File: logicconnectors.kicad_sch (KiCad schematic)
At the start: 31 parts, among them J1 ServoConn, J1 USBC Socket, J10 LHConn, J11 MosTempConn, J12 LogicConn, J2 LogicConn2, J4 ADCConn, J5 HallConn, J6 UartSpi, J7 JTAG, J8 CANConn, U2 USBLC6-2P6, U6 TJA1051T-3

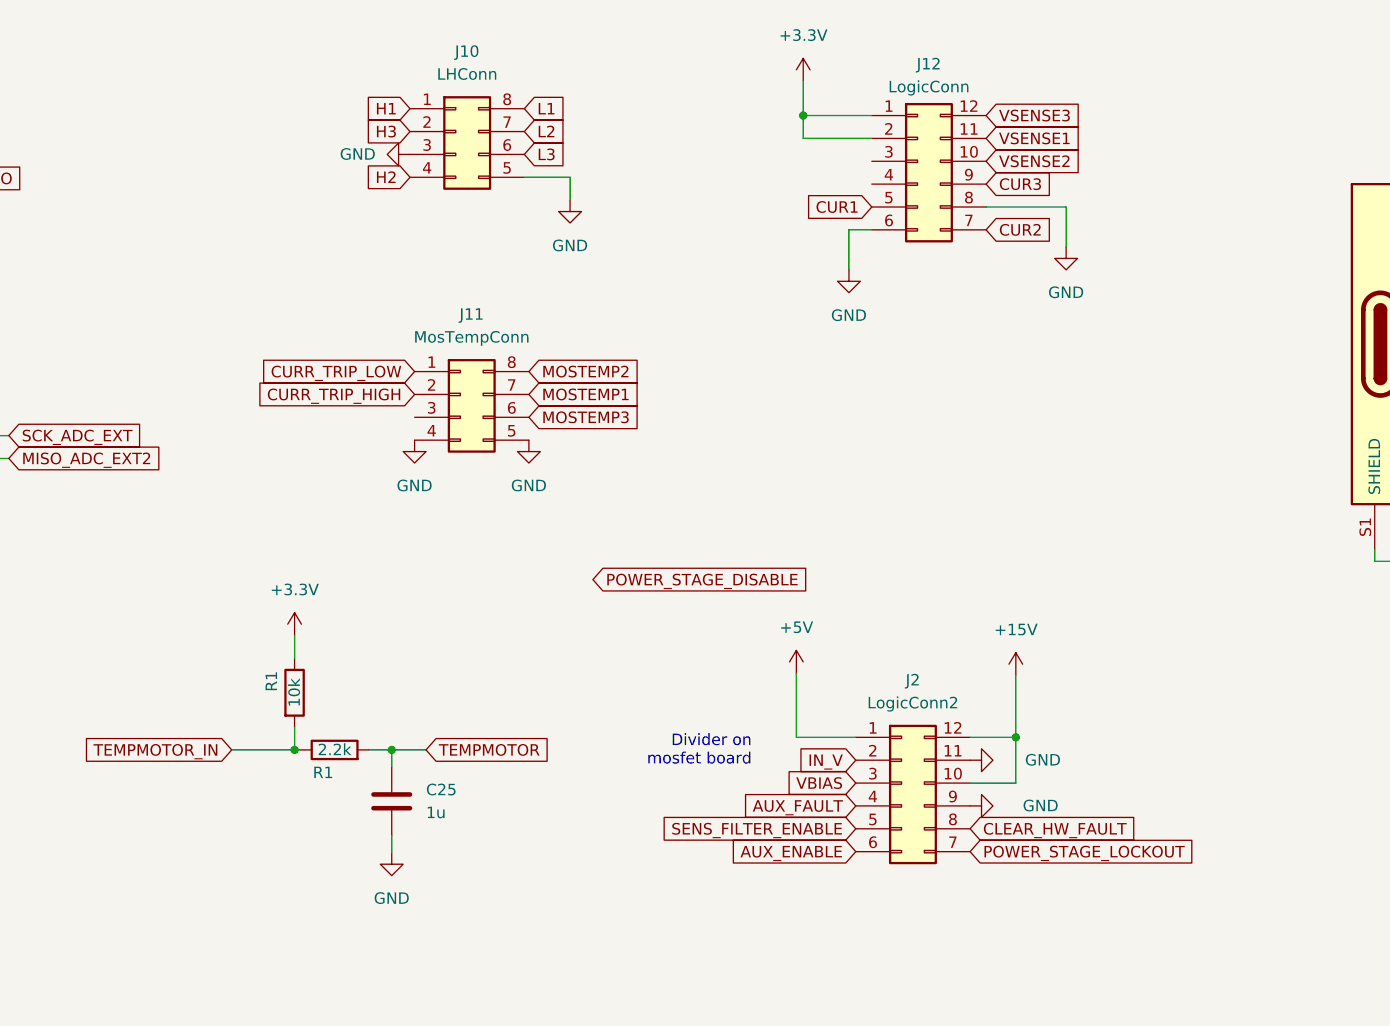
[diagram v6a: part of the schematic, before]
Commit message: routed
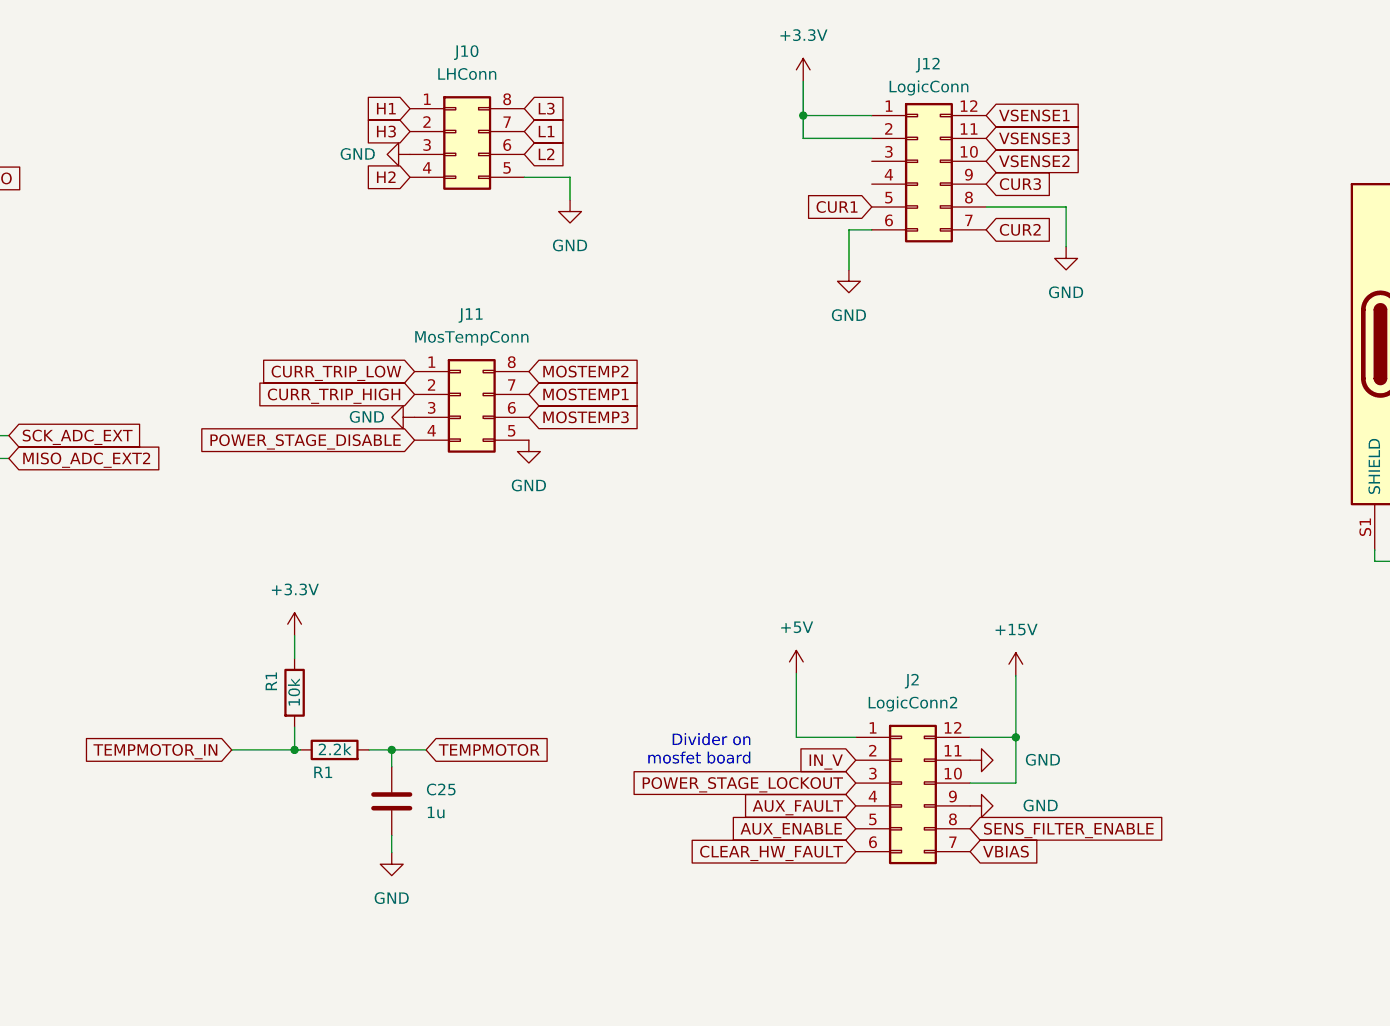
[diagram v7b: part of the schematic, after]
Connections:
- net AUX_ENABLE: now also J2.5 (Pin_5); no longer J2.6 (Pin_6)
- net CLEAR_HW_FAULT: now also J2.6 (Pin_6); no longer J2.8 (Pin_8)
- net GND: now also J11.3 (Pin_3); no longer J11.4 (Pin_4)
- net L1: now also J10.7 (Pin_7); no longer J10.8 (Pin_8)
- net L2: now also J10.6 (Pin_6); no longer J10.7 (Pin_7)
- net L3: now also J10.8 (Pin_8); no longer J10.6 (Pin_6)
- net POWER_STAGE_DISABLE: now also J11.4 (Pin_4)
- net POWER_STAGE_LOCKOUT: now also J2.3 (Pin_3); no longer J2.7 (Pin_7)
- net SENS_FILTER_ENABLE: now also J2.8 (Pin_8); no longer J2.5 (Pin_5)
- net VBIAS: now also J2.7 (Pin_7); no longer J2.3 (Pin_3)
- net VSENSE1: now also J12.12 (Pin_12); no longer J12.11 (Pin_11)
- net VSENSE3: now also J12.11 (Pin_11); no longer J12.12 (Pin_12)

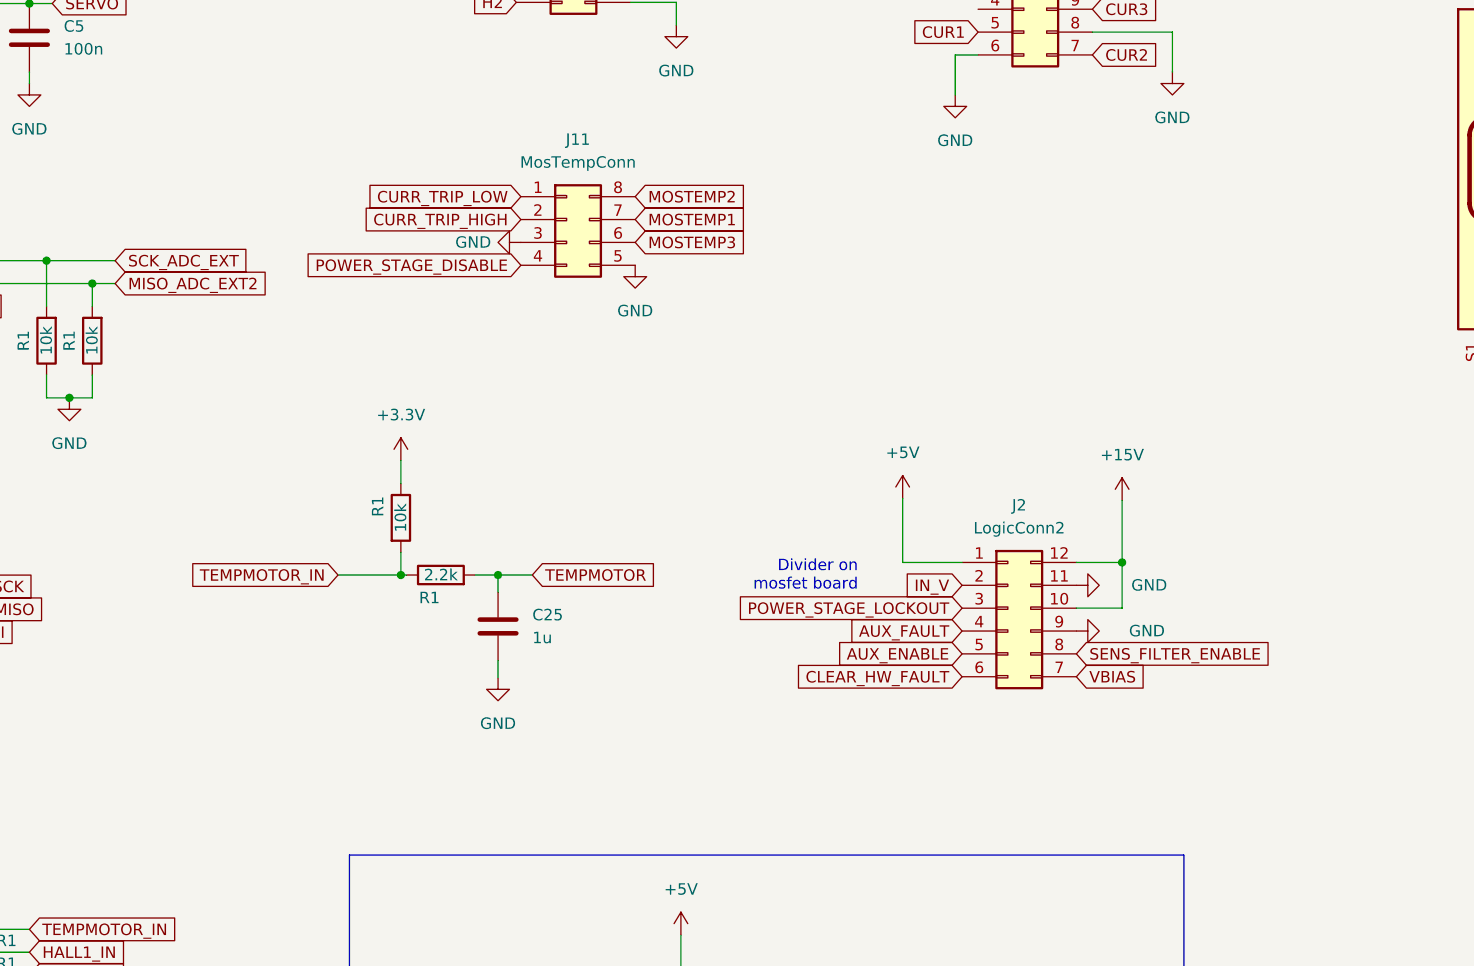
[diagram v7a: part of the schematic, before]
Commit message: driversconnectors
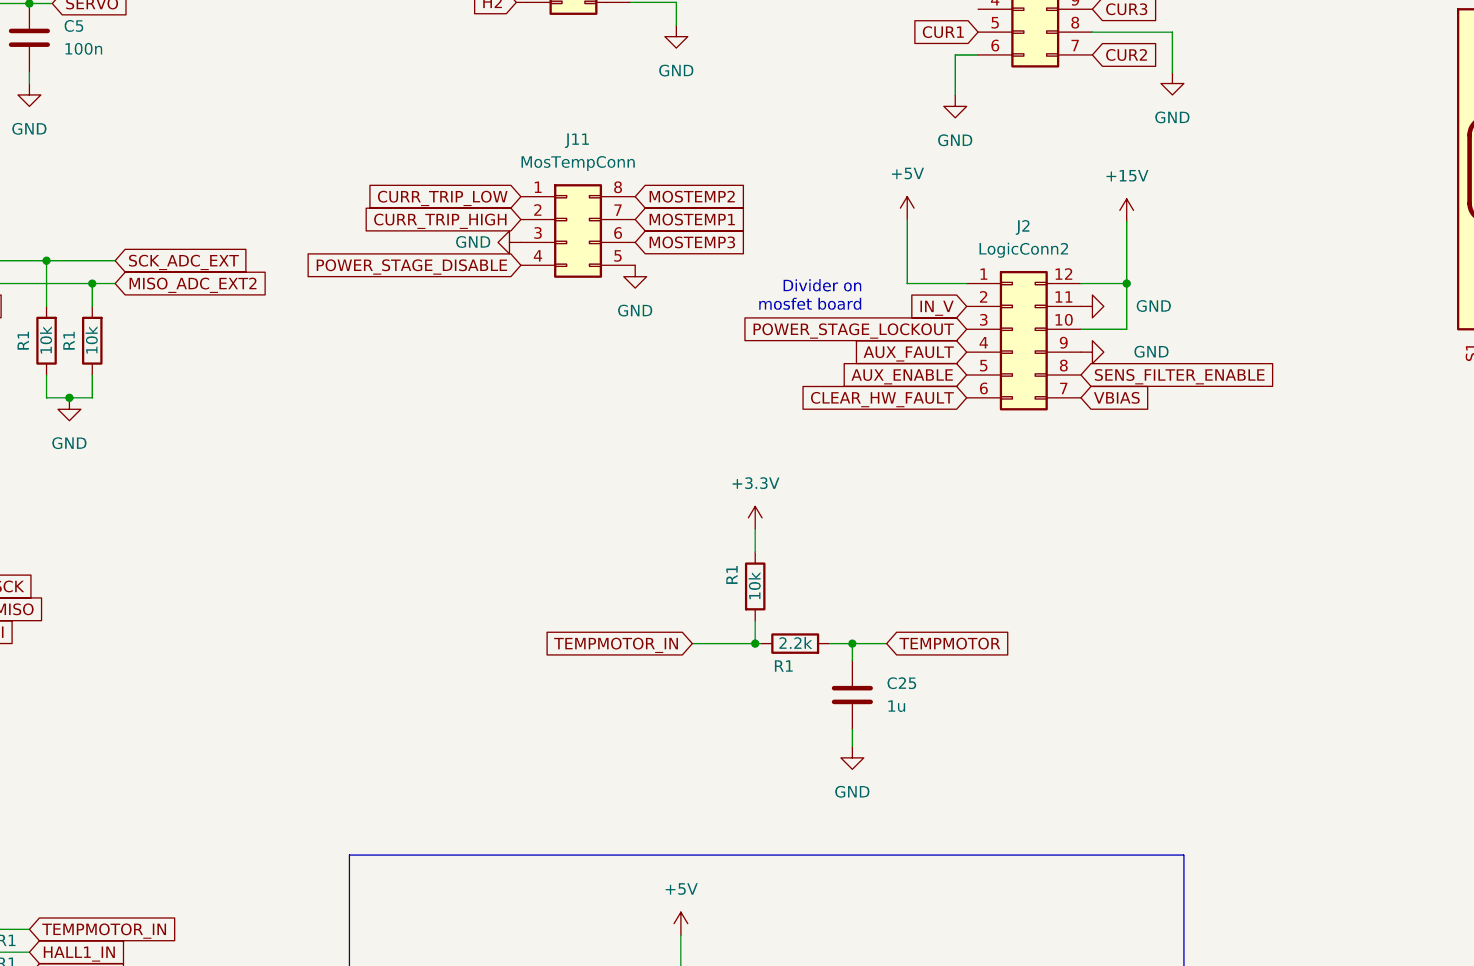
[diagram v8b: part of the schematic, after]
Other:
- moved on the sheet: C25, J2, R1
